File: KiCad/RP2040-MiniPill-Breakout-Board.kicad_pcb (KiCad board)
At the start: 2 copper layers, 52 x 66.5 mm, 27 parts, among them J1 Conn_01x20_Socket, J2 Conn_01x20_Socket, J3 Screw_Terminal_01x20, J4 Screw_Terminal_01x20, Q1 IRLML6402, Q2 IRLML2502, U1 TPS3700

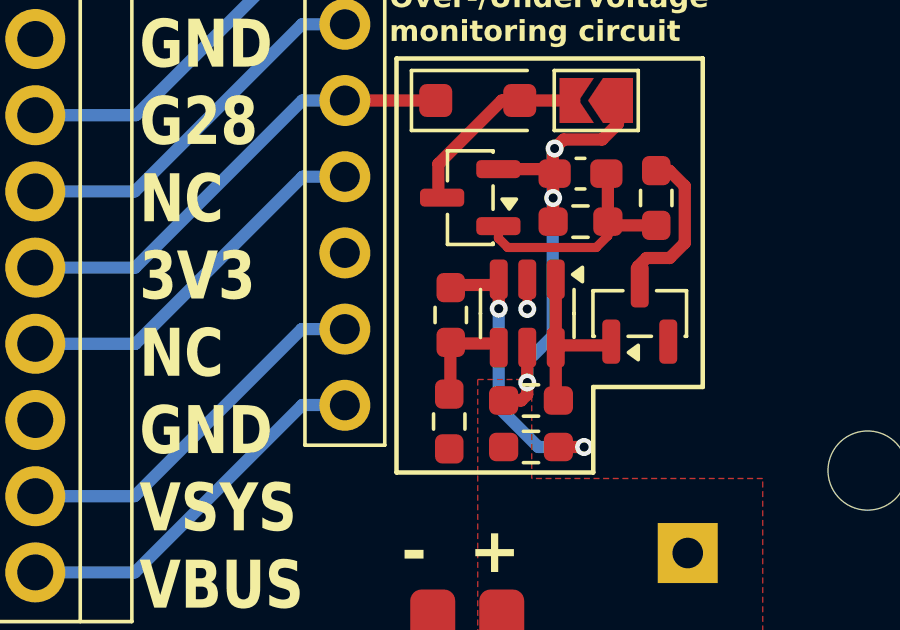
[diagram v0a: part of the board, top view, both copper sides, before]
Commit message: adding some LCSC parts and making some finetuning
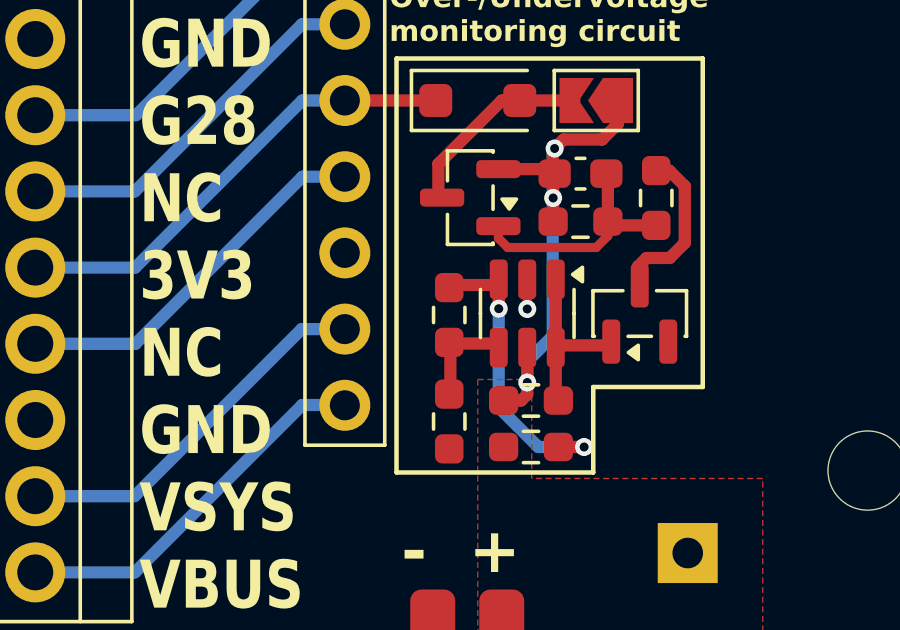
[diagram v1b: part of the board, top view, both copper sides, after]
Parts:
- moved R2 0.05 mm to (136.2, 110.2)
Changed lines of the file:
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@@
 	(footprint "Resistor_SMD:R_0603_1608Metric_Pad0.98x0.95mm_HandSolder"
 		(layer "F.Cu")
-		(at 136.3 110.25 -90)
+		(at 136.25 110.25 -90)
 		(descr "Resistor SMD 0603 (1608 Metric), square (rectangular) end terminal, IPC-7351 nominal with elongated pad for handsoldering. (Body size source: IPC-SM-782 page 72, https://www.pcb-3d.com/wordpress/wp-content/uploads/ipc-sm-782a_amendment_1_and_2.pdf), generated with kicad-footprint-generator")
 		(tags "resistor handsolder")
@@
 			(keep_text_aligned yes)
 		)
-		(gr_text "56"
+		(gr_text "2204.7244"
 			(at 144.2 141.15 0)
 			(layer "Cmts.User")
@@
 			(keep_text_aligned yes)
 		)
-		(gr_text "4.75"
+		(gr_text "187.0079"
 			(at 137.55 63.825 90)
 			(layer "Cmts.User")
@@
 			(keep_text_aligned yes)
 		)
-		(gr_text "43.5"
+		(gr_text "1712.5984"
 			(at 144.2 135.65 0)
 			(layer "Cmts.User")
@@
 			(keep_text_aligned yes)
 		)
-		(gr_text "58"
+		(gr_text "2283.4646"
 			(at 178.05 94.7 90)
 			(layer "Cmts.User")
@@
 			(keep_text_aligned yes)
 		)
-		(gr_text "72"
+		(gr_text "2834.6457"
 			(at 185.15 94.7 90)
 			(layer "Cmts.User")
@@
 			(keep_text_aligned yes)
 		)
-		(gr_text "4.765"
+		(gr_text "187.5984"
 			(at 138.55 120.5675 90)
 			(layer "Cmts.User")
@@
 			(keep_text_aligned yes)
 		)
-		(gr_text "22.86"
+		(gr_text "900"
 			(at 144.2 54.1 0)
 			(layer "Cmts.User")
@@
 	)
 	(segment
-		(start 139.8875 114.65)
-		(end 140.745 114.65)
+		(start 136.3 109.3375)
+		(end 136.25 109.3375)
 		(width 0.4064)
 		(layer "F.Cu")
@@
 	)
 	(segment
-		(start 137.9 109.0625)
-		(end 137.9 110.04)
+		(start 137.7125 109.25)
+		(end 136.3875 109.25)
 		(width 0.4064)
 		(layer "F.Cu")
@@
 	)
 	(segment
-		(start 137.9 109.0625)
-		(end 137.7125 109.25)
+		(start 136.3875 109.25)
+		(end 136.3 109.3375)
 		(width 0.4064)
 		(layer "F.Cu")
@@
 	)
 	(segment
-		(start 136.3875 109.25)
-		(end 136.3 109.3375)
+		(start 139.8875 114.65)
+		(end 140.745 114.65)
 		(width 0.4064)
 		(layer "F.Cu")
@@
 	)
 	(segment
-		(start 137.7125 109.25)
-		(end 136.3875 109.25)
+		(start 137.9 109.0625)
+		(end 137.9 110.04)
+		(width 0.4064)
+		(layer "F.Cu")
+		(net 34)
+	)
+	(segment
+		(start 137.9 109.0625)
+		(end 137.7125 109.25)
 		(width 0.4064)
 		(layer "F.Cu")
@@
 	)
 	(segment
-		(start 136.3375 111.2)
-		(end 136.3 111.1625)
+		(start 136.2875 111.2625)
+		(end 136.3 111.25)
 		(width 0.4064)
 		(layer "F.Cu")
@@
 	)
 	(segment
-		(start 136.25 112.8875)
-		(end 136.2875 112.85)
+		(start 136.3 111.2125)
+		(end 136.25 111.1625)
 		(width 0.4064)
 		(layer "F.Cu")
@@
 	)
 	(segment
-		(start 136.3 111.25)
+		(start 136.3375 111.2)
 		(end 136.3 111.1625)
 		(width 0.4064)
@@
 	)
 	(segment
-		(start 136.2875 111.2625)
-		(end 136.3 111.25)
+		(start 137.7625 111.2)
+		(end 136.3375 111.2)
 		(width 0.4064)
 		(layer "F.Cu")
@@
 	)
 	(segment
-		(start 137.7625 111.2)
-		(end 136.3375 111.2)
+		(start 136.3 111.1625)
+		(end 136.25 111.1625)
 		(width 0.4064)
 		(layer "F.Cu")
@@
 	)
 	(segment
+		(start 136.3 111.25)
+		(end 136.3 111.2125)
+		(width 0.4064)
+		(layer "F.Cu")
+		(net 35)
+	)
+	(segment
 		(start 137.9 111.3375)
 		(end 137.7625 111.2)
 		(width 0.4064)
 		(layer "F.Cu")
+		(net 35)
+	)
+	(segment
+		(start 136.25 112.8875)
+		(end 136.2875 112.85)
+		(width 0.4064)
+		(layer "F.Cu")
